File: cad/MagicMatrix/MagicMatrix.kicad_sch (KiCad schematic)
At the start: 6 parts, among them SW1 Reset, U1 Raspberry Pi Pico

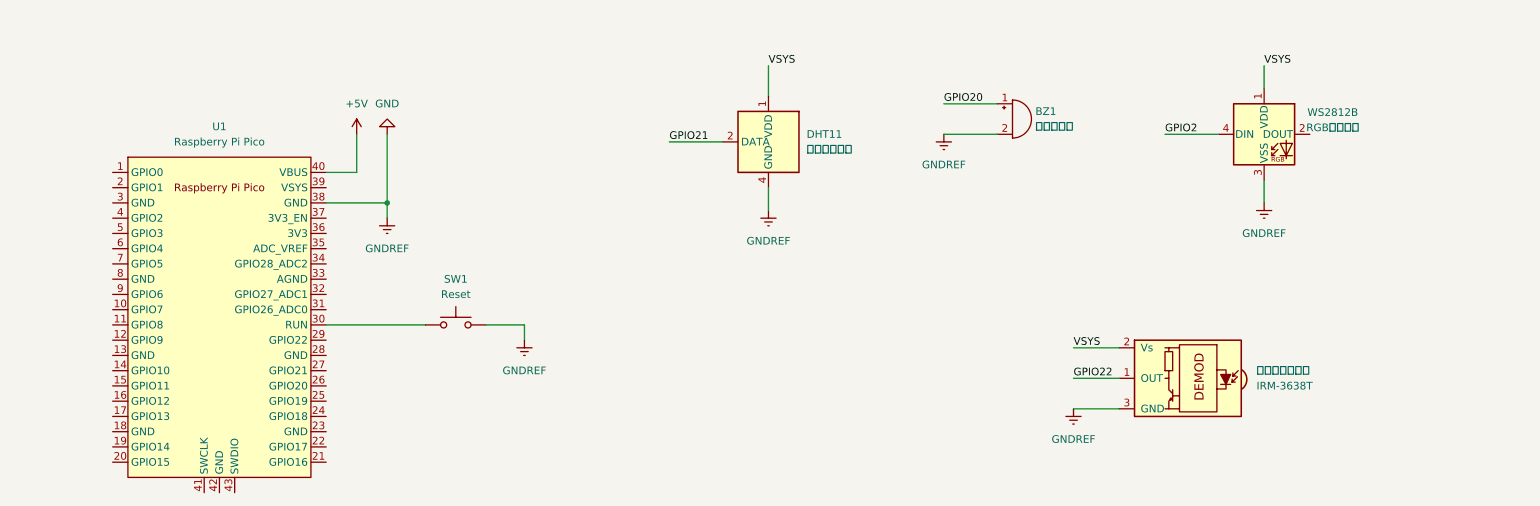
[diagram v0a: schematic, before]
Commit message: update
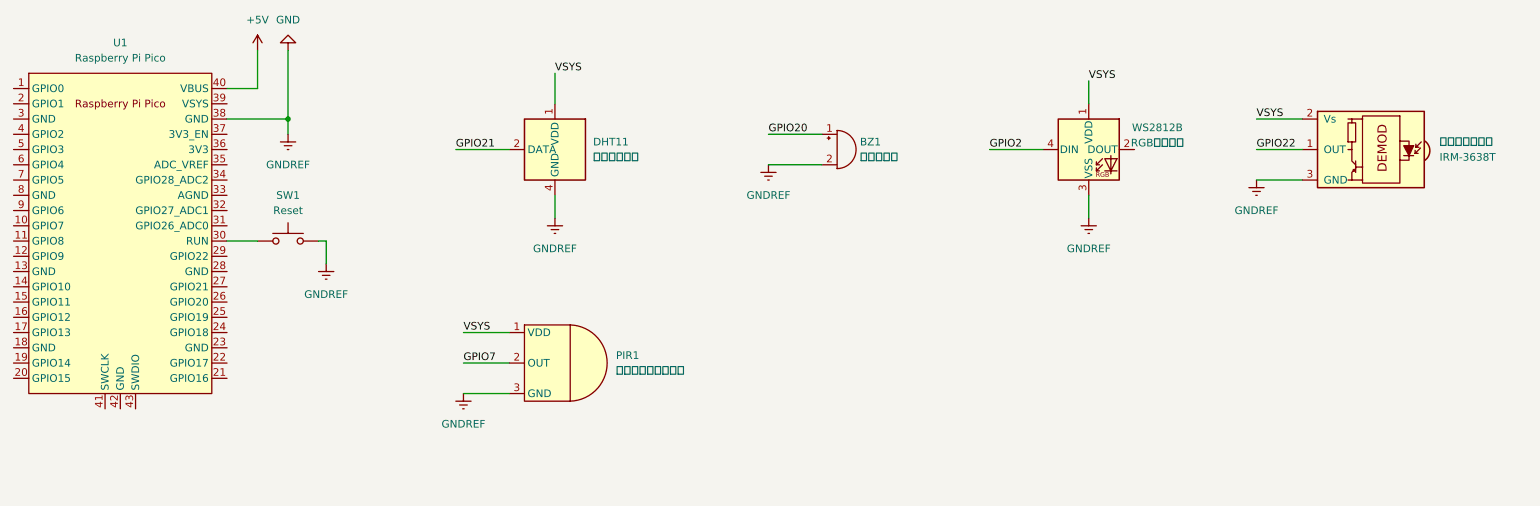
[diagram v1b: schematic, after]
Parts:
- added PIR1: 红外线人体探测模块, symbol MCU_RaspberryPi_and_Boards:PIR
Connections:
- net GND: now also PIR1.3 (GND)
- net VSYS: now also PIR1.1 (VDD)
- new net GPIO7: PIR1.2 (OUT)
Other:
- moved on the sheet: BZ1, IRM-3638T, SW1, U1, WS2812B, 温湿度传感器
